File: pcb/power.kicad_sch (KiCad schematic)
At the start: 10 parts, among them U5 L7805, U6 L7805

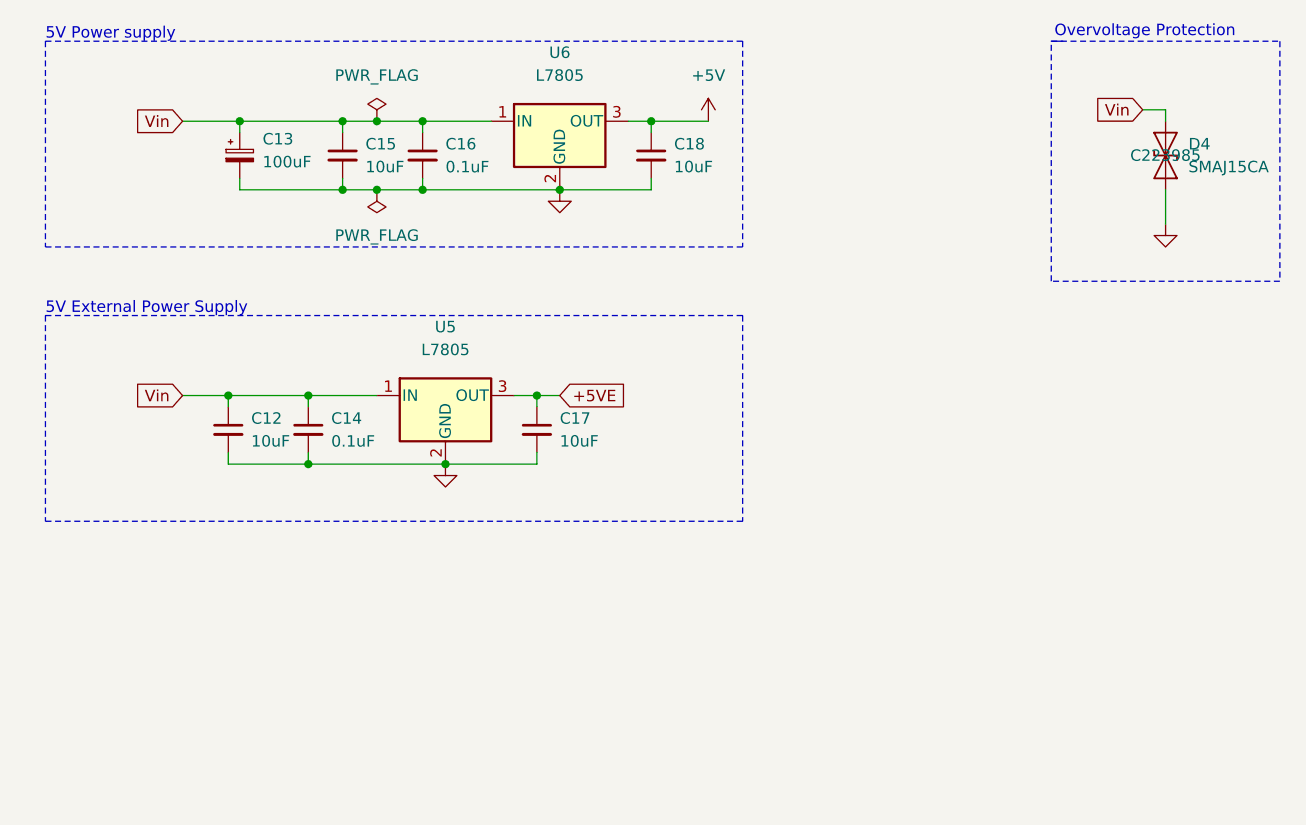
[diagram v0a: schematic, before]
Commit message: Rev 8 MFG artifacts
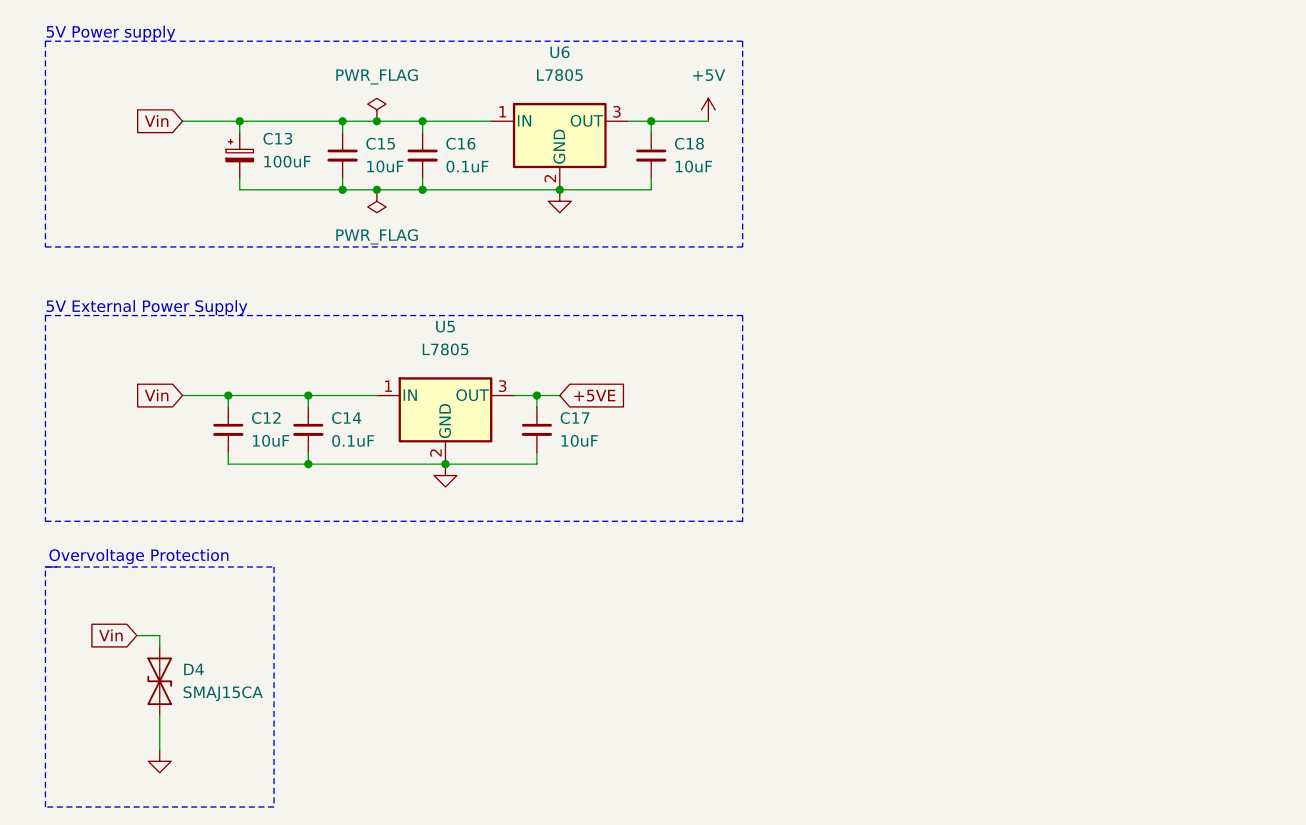
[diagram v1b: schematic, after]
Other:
- moved on the sheet: D4
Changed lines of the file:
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@@
 	(polyline
 		(pts
-			(xy 190.5 40.64) (xy 190.5 67.31)
+			(xy 78.74 99.06) (xy 78.74 125.73)
 		)
 		(stroke
@@
 	(polyline
 		(pts
-			(xy 165.1 40.64) (xy 190.5 40.64)
+			(xy 53.34 99.06) (xy 78.74 99.06)
 		)
 		(stroke
@@
 	(wire
 		(pts
-			(xy 177.8 57.15) (xy 177.8 60.96)
+			(xy 66.04 115.57) (xy 66.04 119.38)
 		)
 		(stroke
@@
 	(polyline
 		(pts
-			(xy 166.37 40.64) (xy 165.1 40.64)
+			(xy 54.61 99.06) (xy 53.34 99.06)
 		)
 		(stroke
@@
 	(polyline
 		(pts
-			(xy 165.1 67.31) (xy 165.1 40.64)
+			(xy 53.34 125.73) (xy 53.34 99.06)
 		)
 		(stroke
@@
 	(wire
 		(pts
-			(xy 177.8 48.26) (xy 177.8 49.53)
+			(xy 66.04 106.68) (xy 66.04 107.95)
 		)
 		(stroke
@@
 	(polyline
 		(pts
-			(xy 190.5 67.31) (xy 165.1 67.31)
+			(xy 78.74 125.73) (xy 53.34 125.73)
 		)
 		(stroke
@@
 	(wire
 		(pts
-			(xy 175.26 48.26) (xy 177.8 48.26)
+			(xy 63.5 106.68) (xy 66.04 106.68)
 		)
 		(stroke
@@
 	(text "Overvoltage Protection"
 		(exclude_from_sim no)
-		(at 175.514 39.624 0)
+		(at 63.754 98.044 0)
 		(effects
 			(font
@@
 	(global_label "Vin"
 		(shape input)
-		(at 175.26 48.26 180)
+		(at 63.5 106.68 180)
 		(fields_autoplaced yes)
 		(effects
@@
 		)
 		(property "Intersheetrefs" "${INTERSHEET_REFS}"
-			(at 170.0045 48.3394 0)
+			(at 58.2445 106.7594 0)
 			(effects
 				(font
@@
 	(symbol
 		(lib_id "power:GND")
-		(at 177.8 60.96 0)
+		(at 66.04 119.38 0)
 		(unit 1)
 		(exclude_from_sim no)
@@
 		(fields_autoplaced yes)
 		(property "Reference" "#PWR059"
-			(at 177.8 67.31 0)
+			(at 66.04 125.73 0)
 			(effects
 				(font
@@
 		)
 		(property "Value" "GND"
-			(at 177.8 66.04 0)
+			(at 66.04 124.46 0)
 			(effects
 				(font
@@
 		)
 		(property "Footprint" ""
-			(at 177.8 60.96 0)
+			(at 66.04 119.38 0)
 			(effects
 				(font
@@
 		)
 		(property "Datasheet" ""
-			(at 177.8 60.96 0)
+			(at 66.04 119.38 0)
 			(effects
 				(font
@@
 		)
 		(property "Description" "Power symbol creates a global label with name \"GND\" , ground"
-			(at 177.8 60.96 0)
+			(at 66.04 119.38 0)
 			(effects
 				(font
@@
 	(symbol
 		(lib_id "Diode:SMAJ15CA")
-		(at 177.8 53.34 90)
+		(at 66.04 111.76 90)
 		(unit 1)
 		(exclude_from_sim no)
@@
 		(on_board yes)
 		(dnp no)
-		(fields_autoplaced yes)
 		(property "Reference" "D4"
-			(at 180.34 52.0699 90)
+			(at 68.58 110.4899 90)
 			(effects
 				(font
@@
 		)
 		(property "Value" "SMAJ15CA"
-			(at 180.34 54.6099 90)
+			(at 68.58 113.0299 90)
 			(effects
 				(font
@@
 		)
 		(property "Footprint" "Diode_SMD:D_SMA"
-			(at 182.88 53.34 0)
+			(at 71.12 111.76 0)
 			(effects
 				(font
@@
 		)
 		(property "Datasheet" "https://www.littelfuse.com/media?resourcetype=datasheets&itemid=75e32973-b177-4ee3-a0ff-cedaf1abdb93&filename=smaj-datasheet"
-			(at 177.8 53.34 0)
+			(at 66.04 111.76 0)
 			(effects
 				(font
@@
 		)
 		(property "Description" "400W bidirectional Transient Voltage Suppressor, 15.0Vr, SMA(DO-214AC)"
-			(at 177.8 53.34 0)
+			(at 66.04 111.76 0)
 			(effects
 				(font
@@
 		)
 		(property "LCSC" "C223985"
-			(at 177.8 53.34 90)
-			(effects
-				(font
-					(size 1.27 1.27)
-				)
-			)
-		)
+			(at 72.39 115.062 90)
+			(effects
+				(font
+					(size 1.27 1.27)
+				)
+				(hide yes)
+			)
+		)
